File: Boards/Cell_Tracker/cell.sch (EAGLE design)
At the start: 26 parts, among them U2 LMR16020

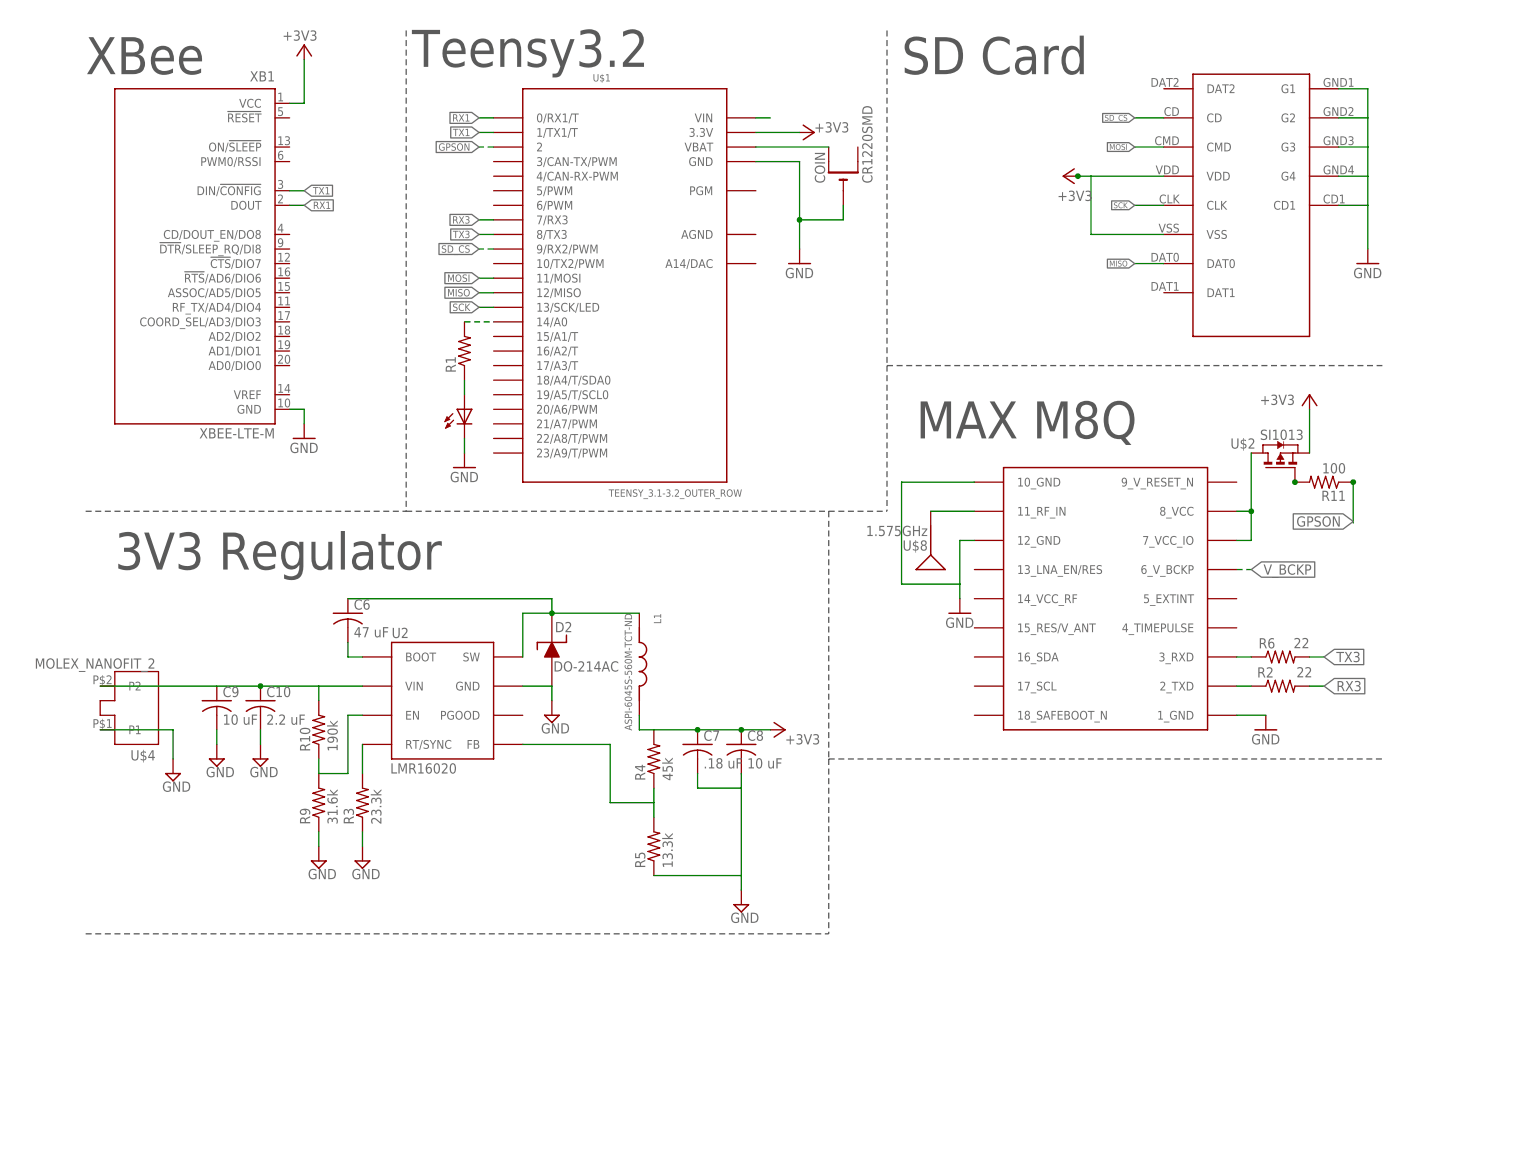
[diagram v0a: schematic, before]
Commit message: All of the changes with CAD and electronics since switching to the microclasp connectors
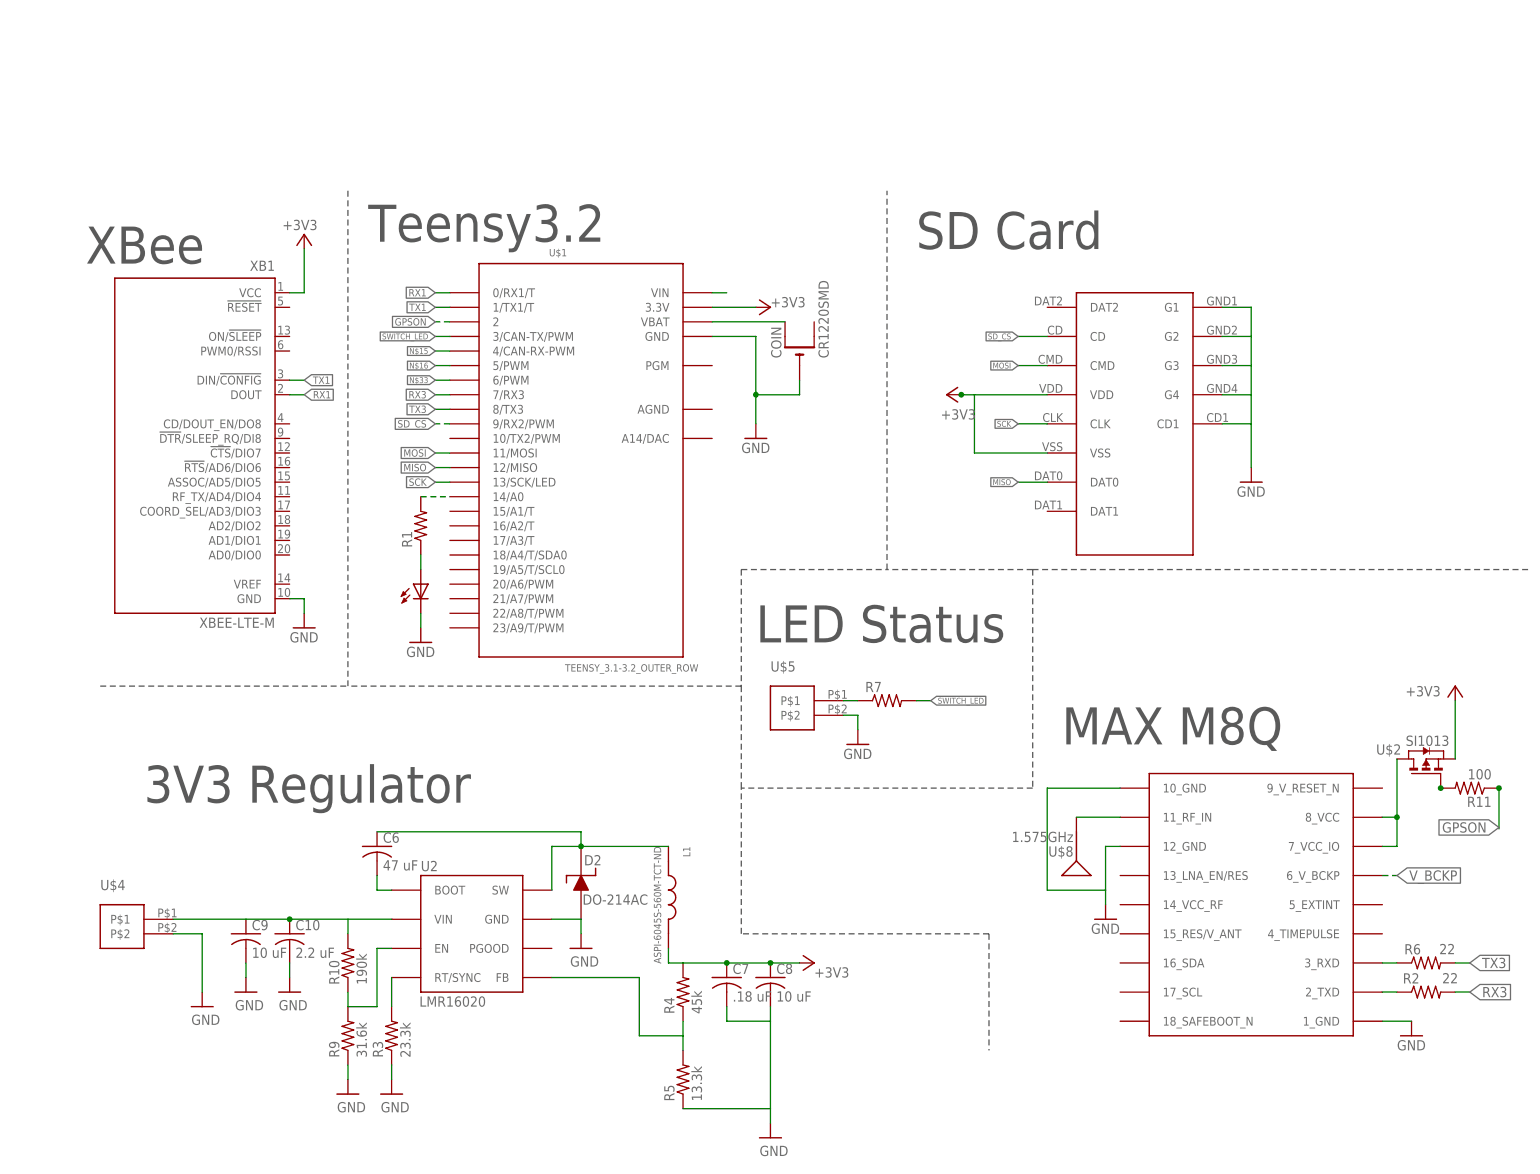
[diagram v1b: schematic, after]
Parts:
- added R7: (no value), resistor:R-US_R0603
- added U$5: (no value), NR_connectors:MICROCLASP
- U$4: value MOLEX_NANOFIT_2 -> (none); device cmdLibs:MOLEX_NANOFIT_2 -> NR_connectors:MICROCLASP
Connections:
- new net N$12: R7.1, U$5.P$1
- new net N$15: U$1.4/CAN-RX-PWM
- new net N$16: U$1.5/PWM
- new net N$33: U$1.6/PWM
- new net SWITCH_LED: R7.2, U$1.3/CAN-TX/PWM
- net GND: now also U$4.P$2, U$5.P$2; no longer U$4.P1
- net VIN: now also U$4.P$1; no longer U$4.P2
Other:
- note added: "LED Status"
- moved on the sheet: C10, C6, C7, C8, C9, COIN, D2, L1, R1, R10, R11, R2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
